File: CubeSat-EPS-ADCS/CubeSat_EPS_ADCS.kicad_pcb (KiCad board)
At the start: 2 copper layers, 92 x 92 mm, 21 parts, among them J1 Conn_01x02_Pin, J2 Conn_01x03_Pin, J3 Conn_01x08_Pin, J4 Screw_Terminal_01x02, J5 Screw_Terminal_01x02, J6 Screw_Terminal_01x02, J7 Screw_Terminal_01x02, U1 DRV8833 Module, U2 DRV8833 Module, U3 Buck_XL4015, U4 Buck_LM2596

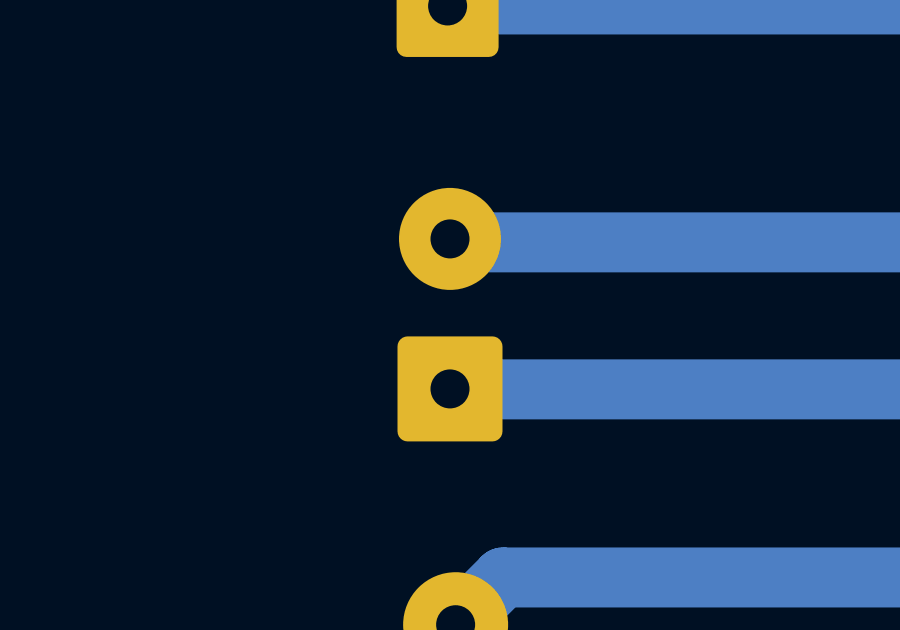
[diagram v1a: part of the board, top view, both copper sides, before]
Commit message: small changes in layout
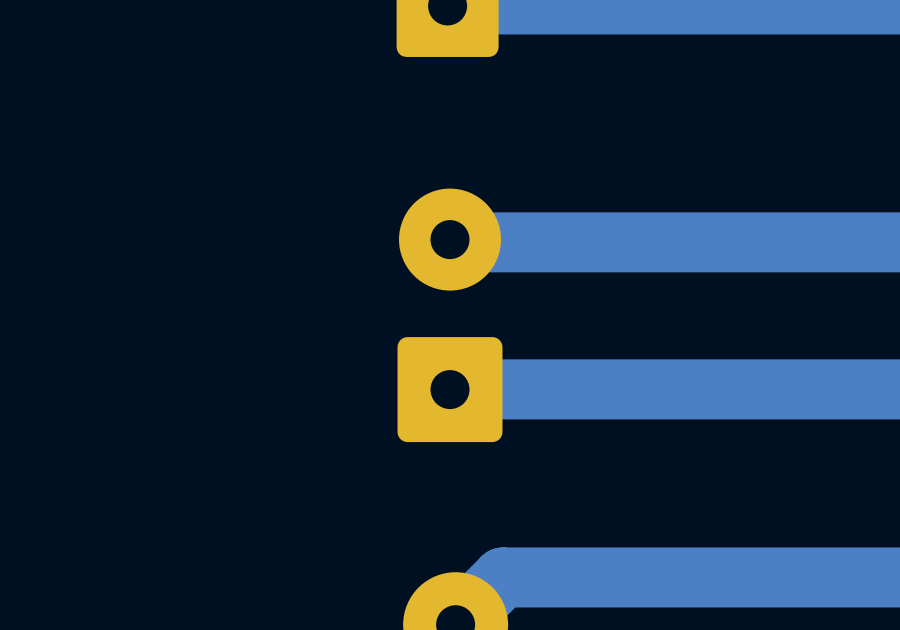
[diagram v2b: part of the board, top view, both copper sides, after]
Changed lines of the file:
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@@
 	(footprint "TerminalBlock_Phoenix:TerminalBlock_Phoenix_MKDS-1,5-2_1x02_P5.00mm_Horizontal"
 		(layer "B.Cu")
-		(at 25.5375 -33.285 90)
+		(at 25.5375 -33.2625 90)
 		(descr "Terminal Block Phoenix MKDS-1,5-2, 2 pins, pitch 5mm, size 10x9.8mm, drill diameter 1.3mm, pad diameter 2.6mm, http://www.farnell.com/datasheets/100425.pdf, script-generated using https://gitlab.com/kicad/libraries/kicad-footprint-generator/-/tree/master/scripts/TerminalBlock_Phoenix")
 		(tags "THT Terminal Block Phoenix MKDS-1,5-2 pitch 5mm size 10x9.8mm drill 1.3mm pad 2.6mm")
